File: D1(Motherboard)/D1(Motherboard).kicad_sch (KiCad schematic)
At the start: 49 parts, among them J1 WR-FPC_0.5mm_ZIF_V, J2 USB_C_Receptacle_USB2.0, J3 B2B-PH-K-S, Q1 NX2301P.215, SW1 CHS-02A, U1 ESP32-S2-MINI-1, U2 ICM-20602, U3 SSD1351, U4 MIC5353-3.3YMT, U5 FAN5331SX, U6 MCP73831-2-OT

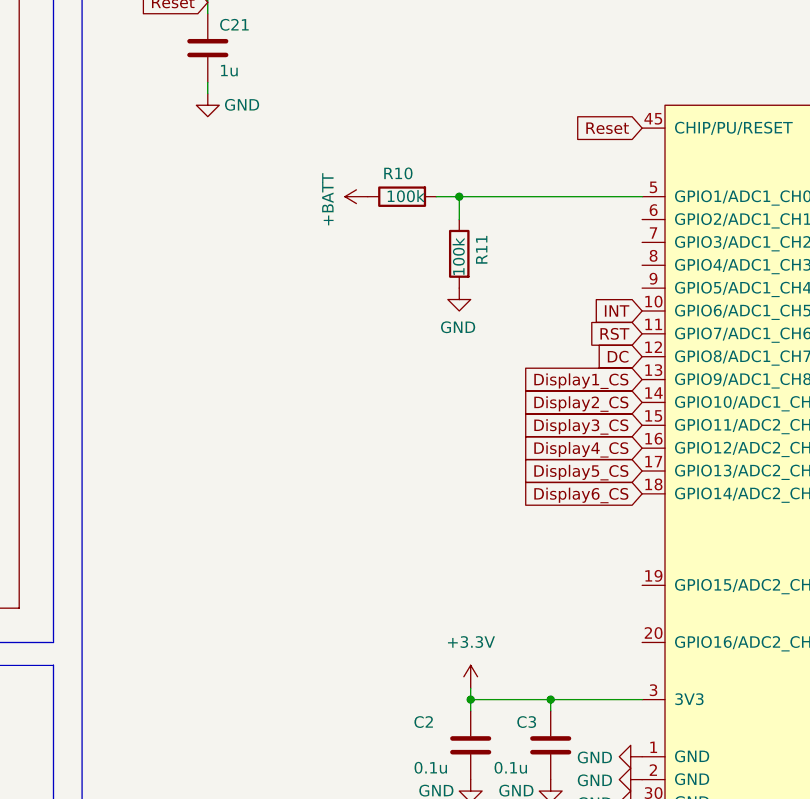
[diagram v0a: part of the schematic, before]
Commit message: More layout work
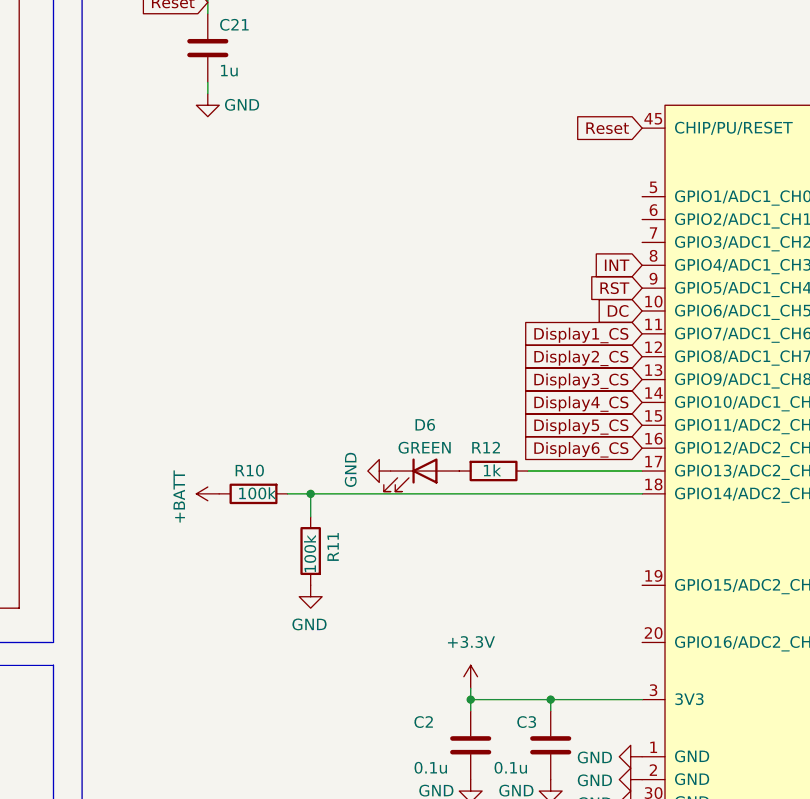
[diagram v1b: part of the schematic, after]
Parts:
- added D6: GREEN, LED_SMD:LED_0603_1608Metric, symbol Device:LED
- added R12: 1k, Resistor_SMD:R_0603_1608Metric, symbol Device:R
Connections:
- net DC: now also U1.10 (GPIO6/ADC1_CH5); no longer U1.12 (GPIO8/ADC1_CH7)
- net Display1_CS: now also U1.11 (GPIO7/ADC1_CH6); no longer U1.13 (GPIO9/ADC1_CH8)
- net Display2_CS: now also U1.12 (GPIO8/ADC1_CH7); no longer U1.14 (GPIO10/ADC1_CH9)
- net Display3_CS: now also U1.13 (GPIO9/ADC1_CH8); no longer U1.15 (GPIO11/ADC2_CH0)
- net Display4_CS: now also U1.14 (GPIO10/ADC1_CH9); no longer U1.16 (GPIO12/ADC2_CH1)
- net Display5_CS: now also U1.15 (GPIO11/ADC2_CH0); no longer U1.17 (GPIO13/ADC2_CH2)
- net Display6_CS: now also U1.16 (GPIO12/ADC2_CH1); no longer U1.18 (GPIO14/ADC2_CH3)
- net GND: now also D6.1 (K)
- net INT: now also U1.8 (GPIO4/ADC1_CH3); no longer U1.10 (GPIO6/ADC1_CH5)
- net RST: now also U1.9 (GPIO5/ADC1_CH4); no longer U1.11 (GPIO7/ADC1_CH6)
- net at R10.2, R11.1: now also U1.18 (GPIO14/ADC2_CH3); no longer U1.5 (GPIO1/ADC1_CH0)
- new net: R12.1, U1.17 (GPIO13/ADC2_CH2)
- new net: D6.2 (A), R12.2
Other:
- moved on the sheet: R10, R11

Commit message: CHECK SOFTWARE OF MULTIPLE SPI DEVICES FIRST
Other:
- note added: "LOOK AT THIS LINK BEFORE DOING ANYMORE WORK TO FIGURE OUT THE SOFTWARE SIDE OF GETTING MULTIPLE DISPLAYS WORKING AT ONCE https://learn.adafruit.com/animated-snake-eyes-bonnet-for-raspberry-pi/software-installation"
- note removed: "CHECK THE CHIP FOR ESP32 AND THE FOOTPRINT"
- note removed: "FIND VALUES OF CAPS INDUCTORS FOR CRYSTAL AND ANTENNA"
- note removed: "GO THROUGH THE HARDWARE DESIGN GUIDES TO SEE IF ALL ASPECTS ARE VALID"
- note removed: "IS ZERO OHM RESISTOR NEEDED FOR THE CRYSTAL???"
- note removed: "WHAT ARE YOU MEANT TO DO WITH PINS OF ANTENNA?"
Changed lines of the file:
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@@
-    (effects (font (size 5 5) (thickness 1) bold italic) (justify left bottom))
-  )
-  (text "GO THROUGH THE HARDWARE DESIGN GUIDES\nTO SEE IF ALL ASPECTS ARE VALID"
-    (at 422.91 198.12 0)
     (effects (font (size 5 5) (thickness 1) bold italic) (justify left bottom))
   )
@@
     (effects (font (size 5 5) (thickness 1) bold italic) (justify left bottom))
   )
-  (text "WHAT ARE YOU MEANT TO DO WITH PINS OF ANTENNA?" (at 422.91 45.72 0)
+  (text "https://shop.pimoroni.com/products/adafruit-esp32-s2-feather-2-mb-psram-and-stemma-qt-qwiic"
+    (at 2.54 34.29 0)
     (effects (font (size 5 5) (thickness 1) bold italic) (justify left bottom))
   )
-  (text "IS ZERO OHM RESISTOR NEEDED FOR THE CRYSTAL???" (at 422.91 130.81 0)
-    (effects (font (size 5 5) (thickness 1) bold italic) (justify left bottom))
-  )
-  (text "https://shop.pimoroni.com/products/adafruit-esp32-s2-feather-2-mb-psram-and-stemma-qt-qwiic"
-    (at 2.54 34.29 0)
+  (text "LOOK AT THIS LINK BEFORE DOING ANYMORE WORK TO FIGURE OUT THE SOFTWARE SIDE OF GETTING MULTIPLE DISPLAYS WORKING AT ONCE\nhttps://learn.adafruit.com/animated-snake-eyes-bonnet-for-raspberry-pi/software-installation"
+    (at -27.94 133.35 0)
     (effects (font (size 5 5) (thickness 1) bold italic) (justify left bottom))
   )
@@
     (effects (font (size 5 5) (thickness 1) bold italic) (justify left bottom))
   )
-  (text "CHECK THE CHIP FOR ESP32 AND THE FOOTPRINT" (at 421.64 8.89 0)
-    (effects (font (size 5 5) (thickness 1) bold italic) (justify left bottom))
-  )
-  (text "FIND VALUES OF CAPS INDUCTORS FOR CRYSTAL AND ANTENNA"
-    (at 422.91 27.94 0)
-    (effects (font (size 5 5) (thickness 1) bold italic) (justify left bottom))
-  )

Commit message: Some possible links to solutions
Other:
- note added: "TRY OTHER SSD1351 LIBRARIES TO SEE WHAT ELSE YOU CAN DO TO GET MULTIPLE DISPLAYS WORKING"
- note added: "http://adafruit.github.io/Adafruit-SSD1351-library/html/class_adafruit___s_s_d1351.html#ab6e1ac8ed42279367c60977c8bf3fb4f https://github.com/olikraus/ucglib/wiki"
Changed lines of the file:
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@@
+    (effects (font (size 5 5) (thickness 1) bold italic) (justify left bottom))
+  )
+  (text "TRY OTHER SSD1351 LIBRARIES TO SEE WHAT ELSE YOU CAN DO TO GET MULTIPLE DISPLAYS WORKING"
+    (at 10.16 232.41 0)
     (effects (font (size 5 5) (thickness 1) bold italic) (justify left bottom))
   )
@@
     (effects (font (size 5 5) (thickness 1) bold italic) (justify left bottom))
   )
+  (text "http://adafruit.github.io/Adafruit-SSD1351-library/html/class_adafruit___s_s_d1351.html#ab6e1ac8ed42279367c60977c8bf3fb4f\n\nhttps://github.com/olikraus/ucglib/wiki"
+    (at 10.16 255.27 0)
+    (effects (font (size 5 5) (thickness 1) bold italic) (justify left bottom))
+  )
